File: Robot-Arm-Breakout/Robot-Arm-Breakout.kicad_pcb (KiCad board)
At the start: 2 copper layers, 43.2 x 116.8 mm, 16 parts, among them J1 Pico-Parrallel, J10 Conn_01x03_Pin, J2 Conn_01x03_Pin, J3 Conn_01x03_Pin, J4 Conn_01x03_Pin, J5 Conn_01x03_Socket, J6 Conn_01x03_Socket, J7 Conn_01x03_Socket, J8 Conn_01x03_Pin, J9 Conn_01x03_Pin

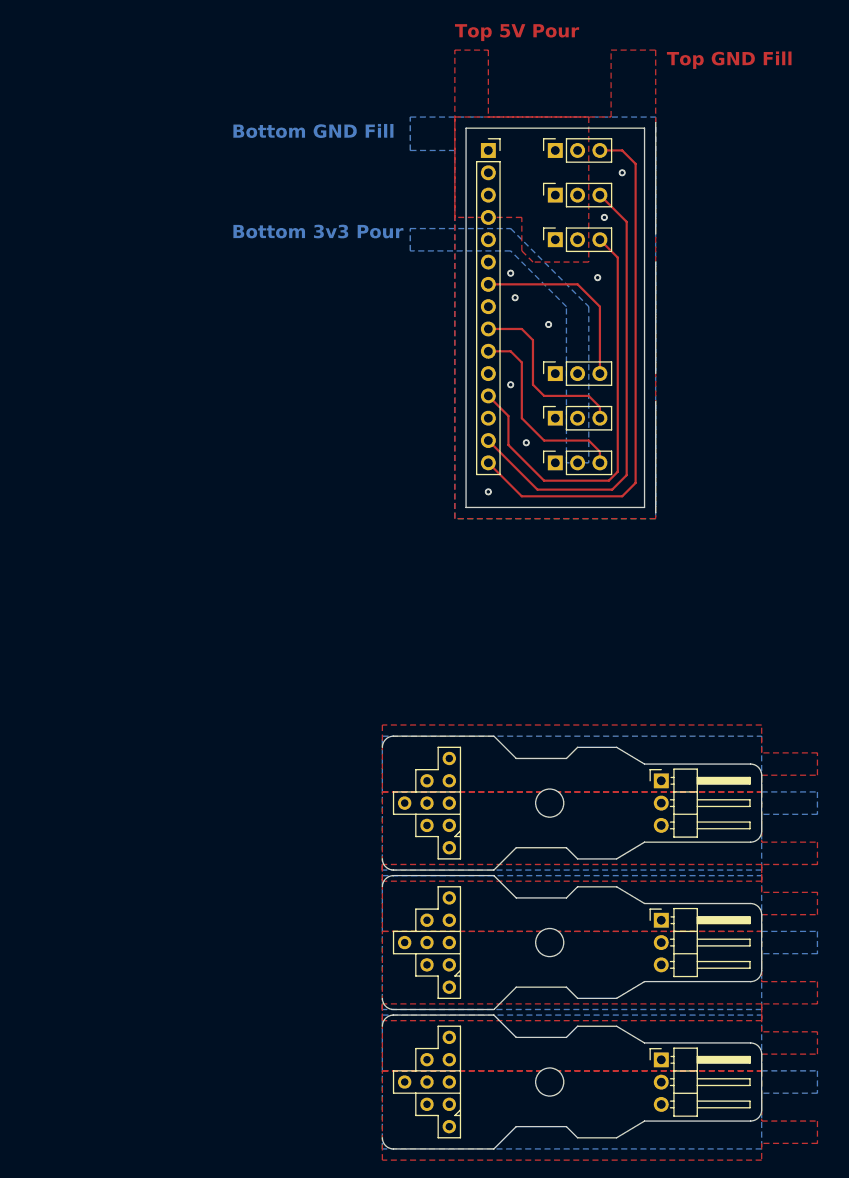
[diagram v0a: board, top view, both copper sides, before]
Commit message: All silkscreen done
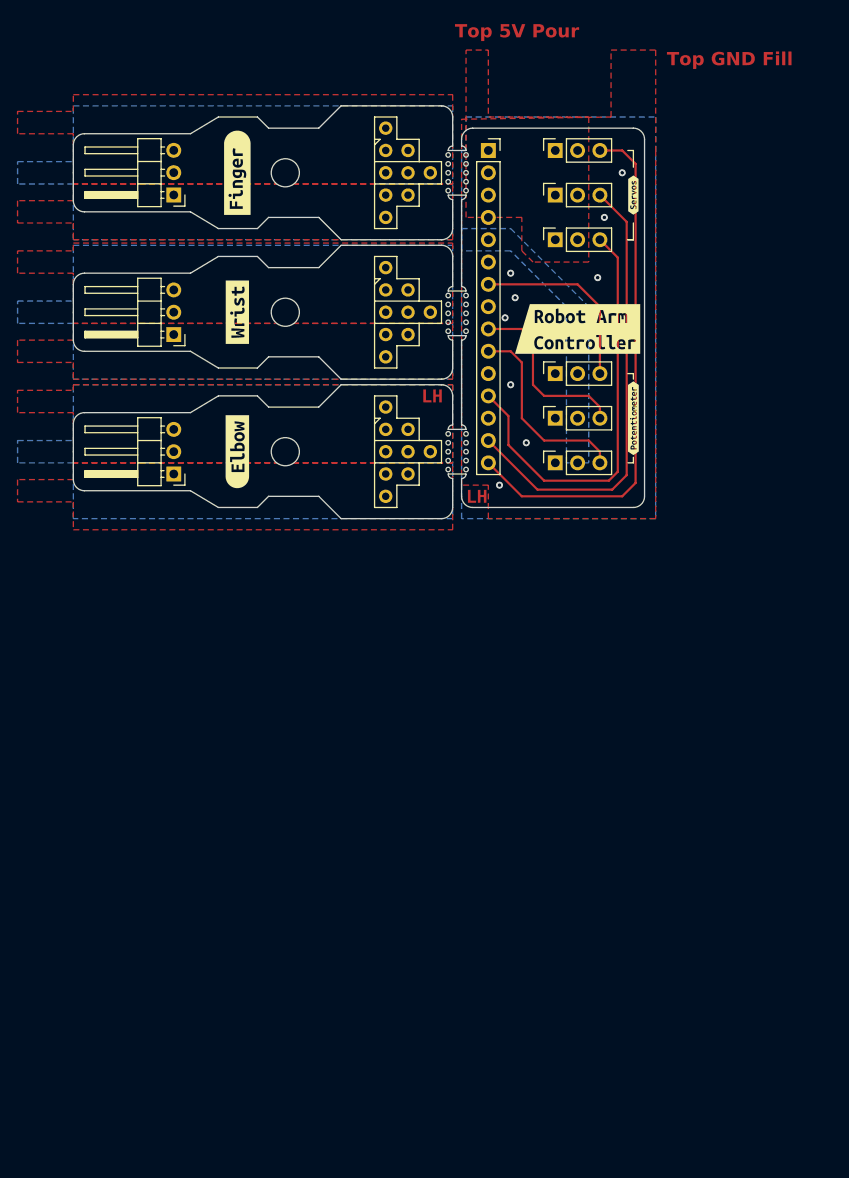
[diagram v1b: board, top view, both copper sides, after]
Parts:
- added kibuzzard-65757C16: G***, kibuzzard-65757C16, F.Cu at (64.8, 79.7)
- added kibuzzard-65757C1E: G***, kibuzzard-65757C1E, F.Cu at (64.8, 54.3)
- added kibuzzard-65757EFB: G***, kibuzzard-65757EFB, F.Cu at (58.4, 69.5)
- added kibuzzard-6575800A: G***, kibuzzard-6575800A, F.Cu at (19.7, 51.8)
- added kibuzzard-65758041: G***, kibuzzard-65758041, F.Cu at (19.7, 83.5)
- added kibuzzard-65758048: G***, kibuzzard-65758048, F.Cu at (19.7, 67.6)
- added kibuzzard-657581BB: G***, kibuzzard-657581BB, B.Cu at (57.8, 88.0)
- added kibuzzard-65758245: G***, kibuzzard-65758245, F.Cu at (47.0, 88.6)
- added kibuzzard-65758245: G***, kibuzzard-65758245, F.Cu at (41.9, 77.2)
- moved J10 113.0 mm to (12.4, 54.3), turned to 180 degrees
- moved RV3 108.8 mm to (36.6, 49.2), turned to 0 degrees
- moved H3 107.8 mm to (25.1, 51.8), turned to 180 degrees
- moved J9 86.8 mm to (12.4, 70.2), turned to 180 degrees
- moved H2 77.8 mm to (25.1, 67.6), turned to 180 degrees
- moved RV2 77.2 mm to (36.6, 65.1), turned to 0 degrees
- moved J8 65.6 mm to (12.4, 86.1), turned to 180 degrees
- moved H1 50.1 mm to (25.1, 83.5), turned to 0 degrees
- moved RV1 45.7 mm to (36.6, 81.0), turned to 0 degrees
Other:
- board size 43.2 x 116.8 mm -> 65 x 47 mm
- board text removed: "Bottom 3v3 Pour"
- board text removed: "Bottom GND Fill"
